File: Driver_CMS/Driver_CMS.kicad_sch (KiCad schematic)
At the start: 24 parts, among them J1 Screw_Terminal_01x04, J2 Screw_Terminal_01x04, J3 Screw_Terminal_01x03, U1 L298P

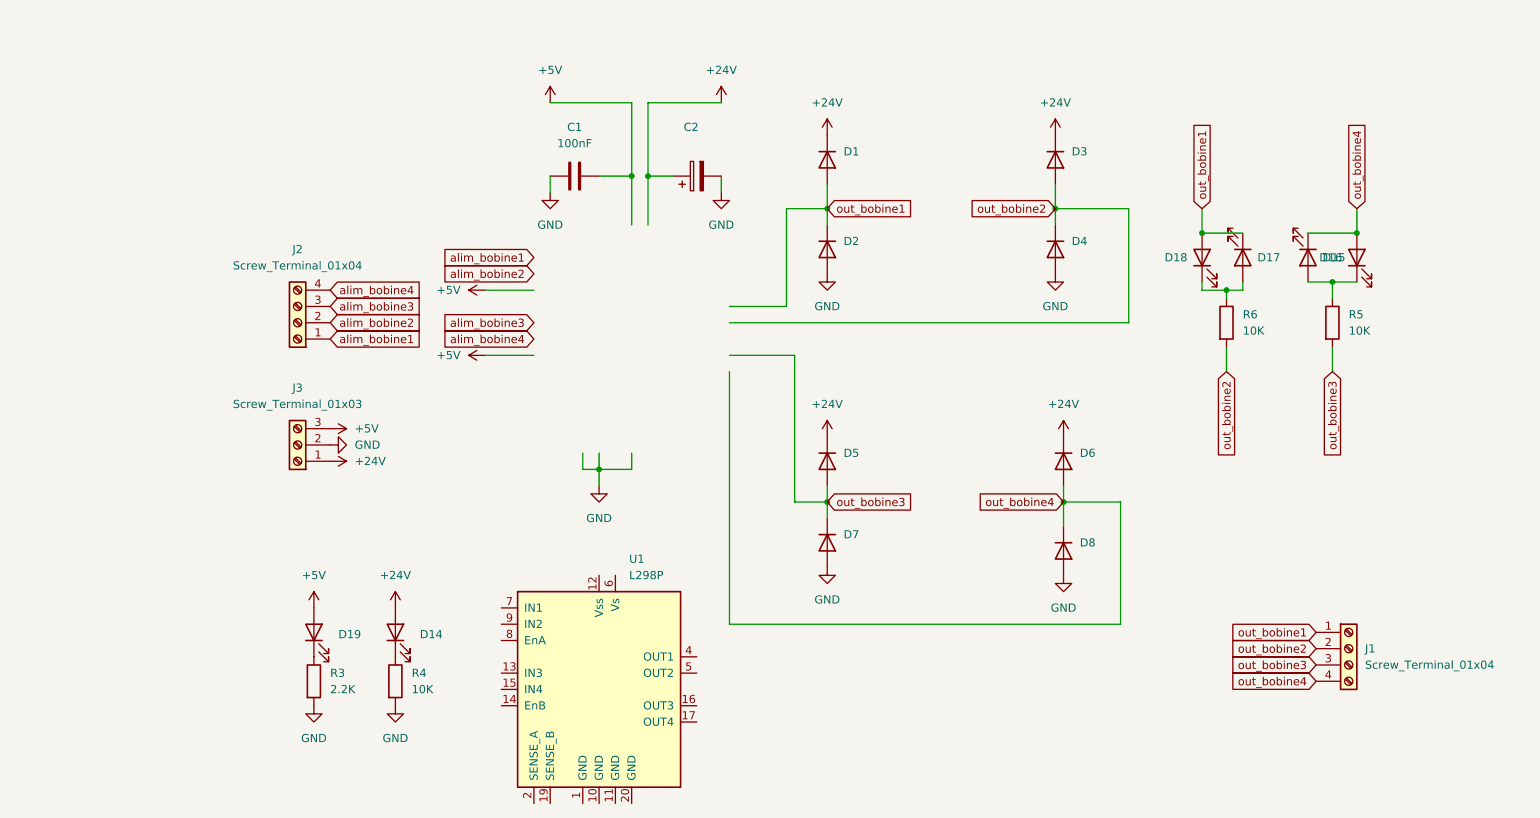
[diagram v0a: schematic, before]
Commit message: Driver CMS DRC OK
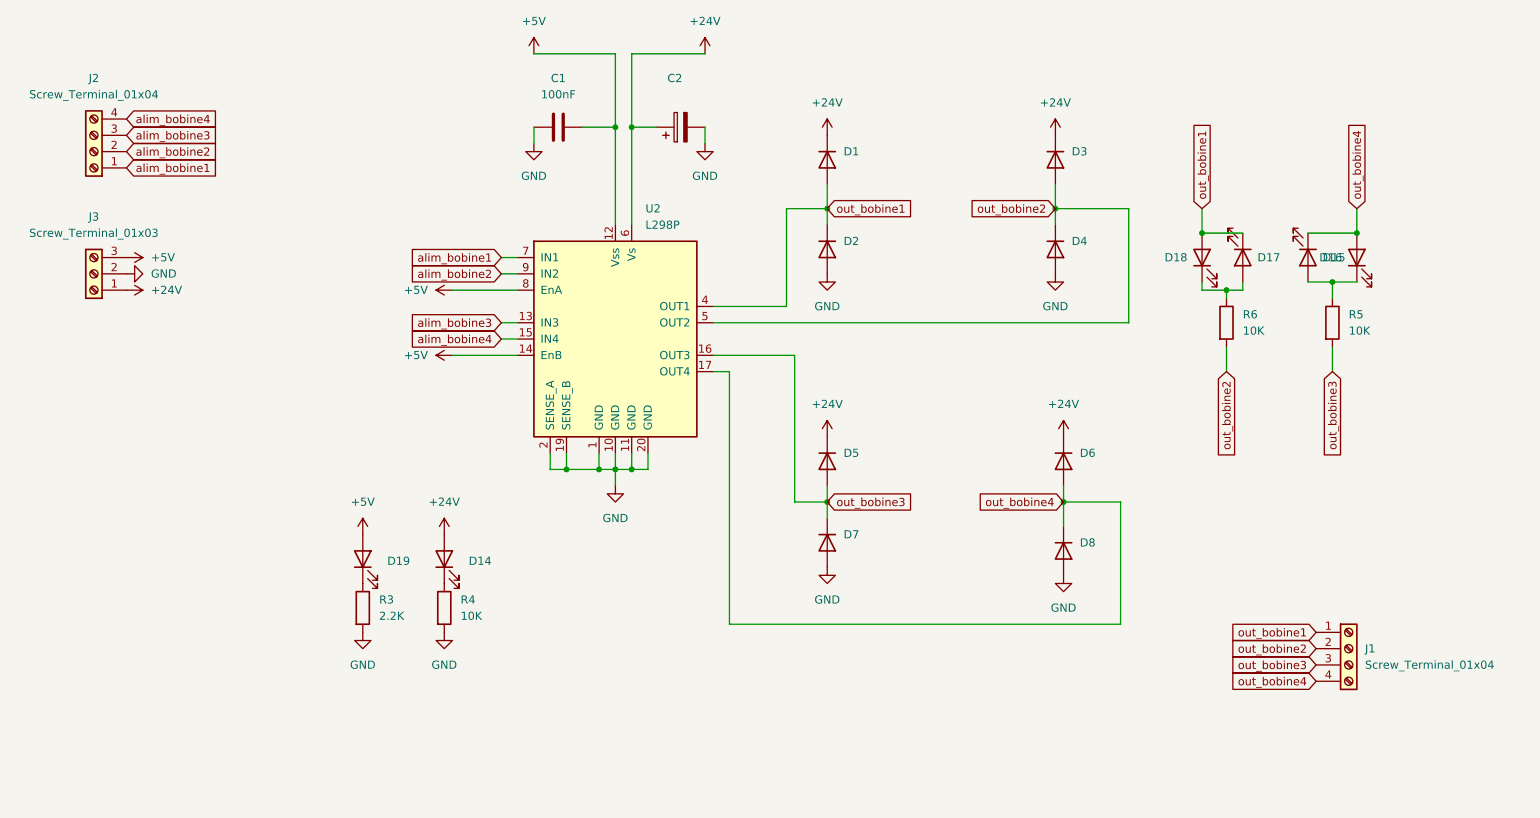
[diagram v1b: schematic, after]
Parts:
- removed U1: L298P, symbol Driver_Motor:L298P
- added U2: L298P, Package_SO:HSOP-20-1EP_11.0x15.9mm_P1.27mm_SlugDown, symbol Driver_Motor:L298P
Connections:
- net +24V: now also U2.6 (Vs)
- net +5V: now also U2.12 (Vss), U2.14 (EnB), U2.8 (EnA)
- net GND: now also U2.1 (GND), U2.10 (GND), U2.11 (GND), U2.19 (SENSE_B), U2.2 (SENSE_A), U2.20 (GND)
- net alim_bobine1: now also U2.7 (IN1)
- net alim_bobine2: now also U2.9 (IN2)
- net alim_bobine3: now also U2.13 (IN3)
- net alim_bobine4: now also U2.15 (IN4)
- net out_bobine1: now also U2.4 (OUT1)
- net out_bobine2: now also U2.5 (OUT2)
- net out_bobine3: now also U2.16 (OUT3)
- net out_bobine4: now also U2.17 (OUT4)
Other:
- moved on the sheet: C1, C2, D14, D19, J2, J3, R3, R4
